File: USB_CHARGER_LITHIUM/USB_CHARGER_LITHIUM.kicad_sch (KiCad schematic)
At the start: 18 parts, among them J1 USB4135, J2 Conn_01x02, J3 Conn_01x02, U1 TP5000X-4.2-ESOP8

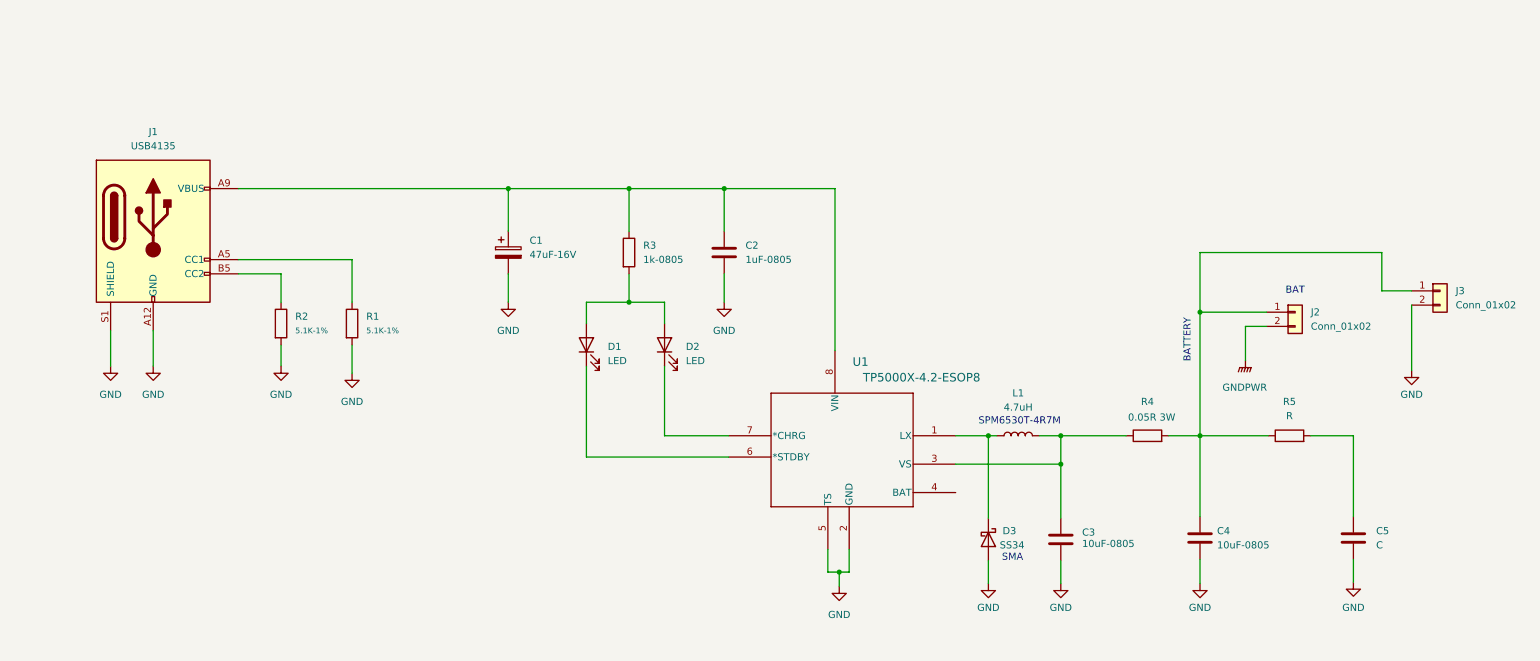
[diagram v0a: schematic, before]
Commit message: Finished Schematic
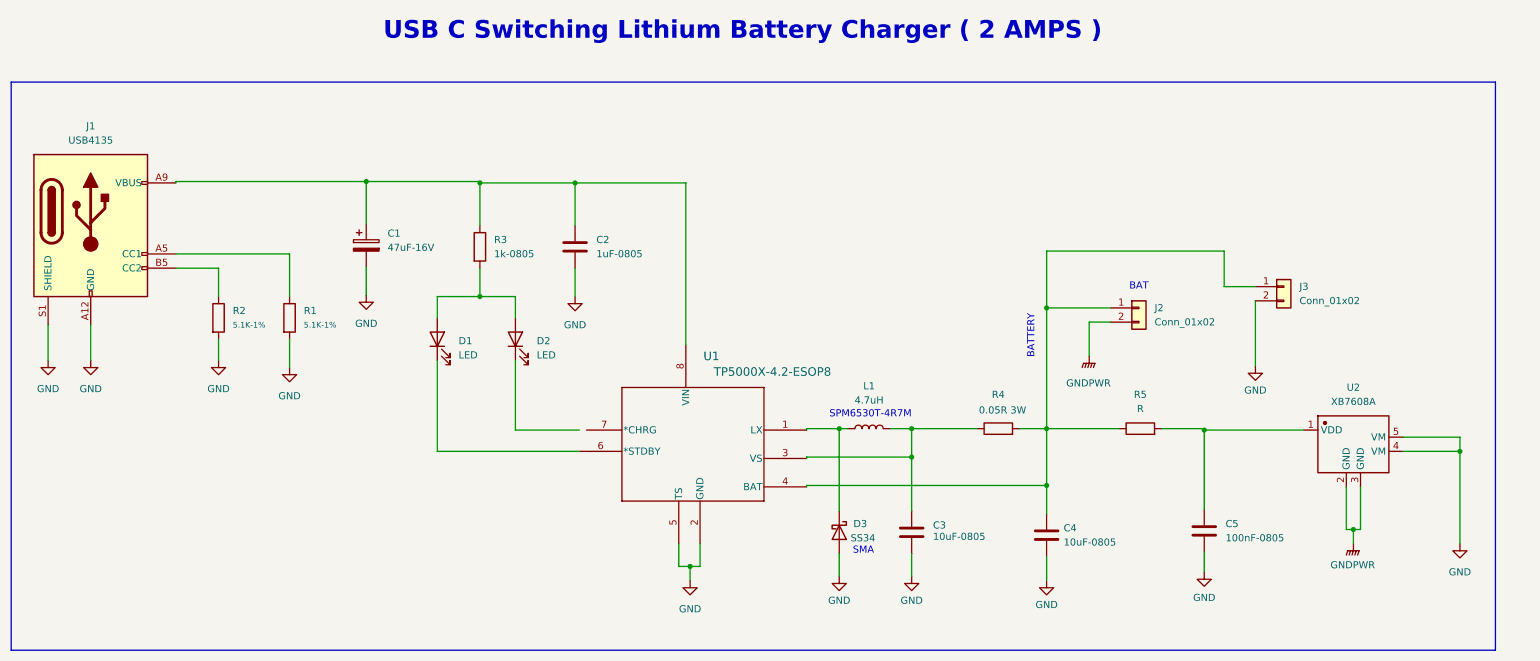
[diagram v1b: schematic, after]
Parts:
- added U2: XB7608A, symbol XB7608A:XB7608A
- C5: value C -> 100nF-0805
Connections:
- net GND: now also U2.4 (VM), U2.5 (VM)
- net GNDPWR: now also U2.2 (GND), U2.3 (GND)
- net at C4.1, J2.1 (Pin_1), J3.1 (Pin_1)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: now also U1.4 (BAT)
- net at C5.1, R5.2: now also U2.1 (VDD)
- net at D2.1 (K): no longer U1.7 (*CHRG)
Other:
- note added: "USB C Switching Lithium Battery Charger ( 2 AMPS )"
- company: (none) -> VICTOR ROSALES
- title: (none) -> USB C Lithium Battery Charger (2AMP)
- moved on the sheet: C1, C2, C3, C4, C5, D1, D2, D3, J1, J2, J3, L1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
